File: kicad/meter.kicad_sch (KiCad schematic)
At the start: 10 parts, among them U10 MAX7219, U9 MAX7219

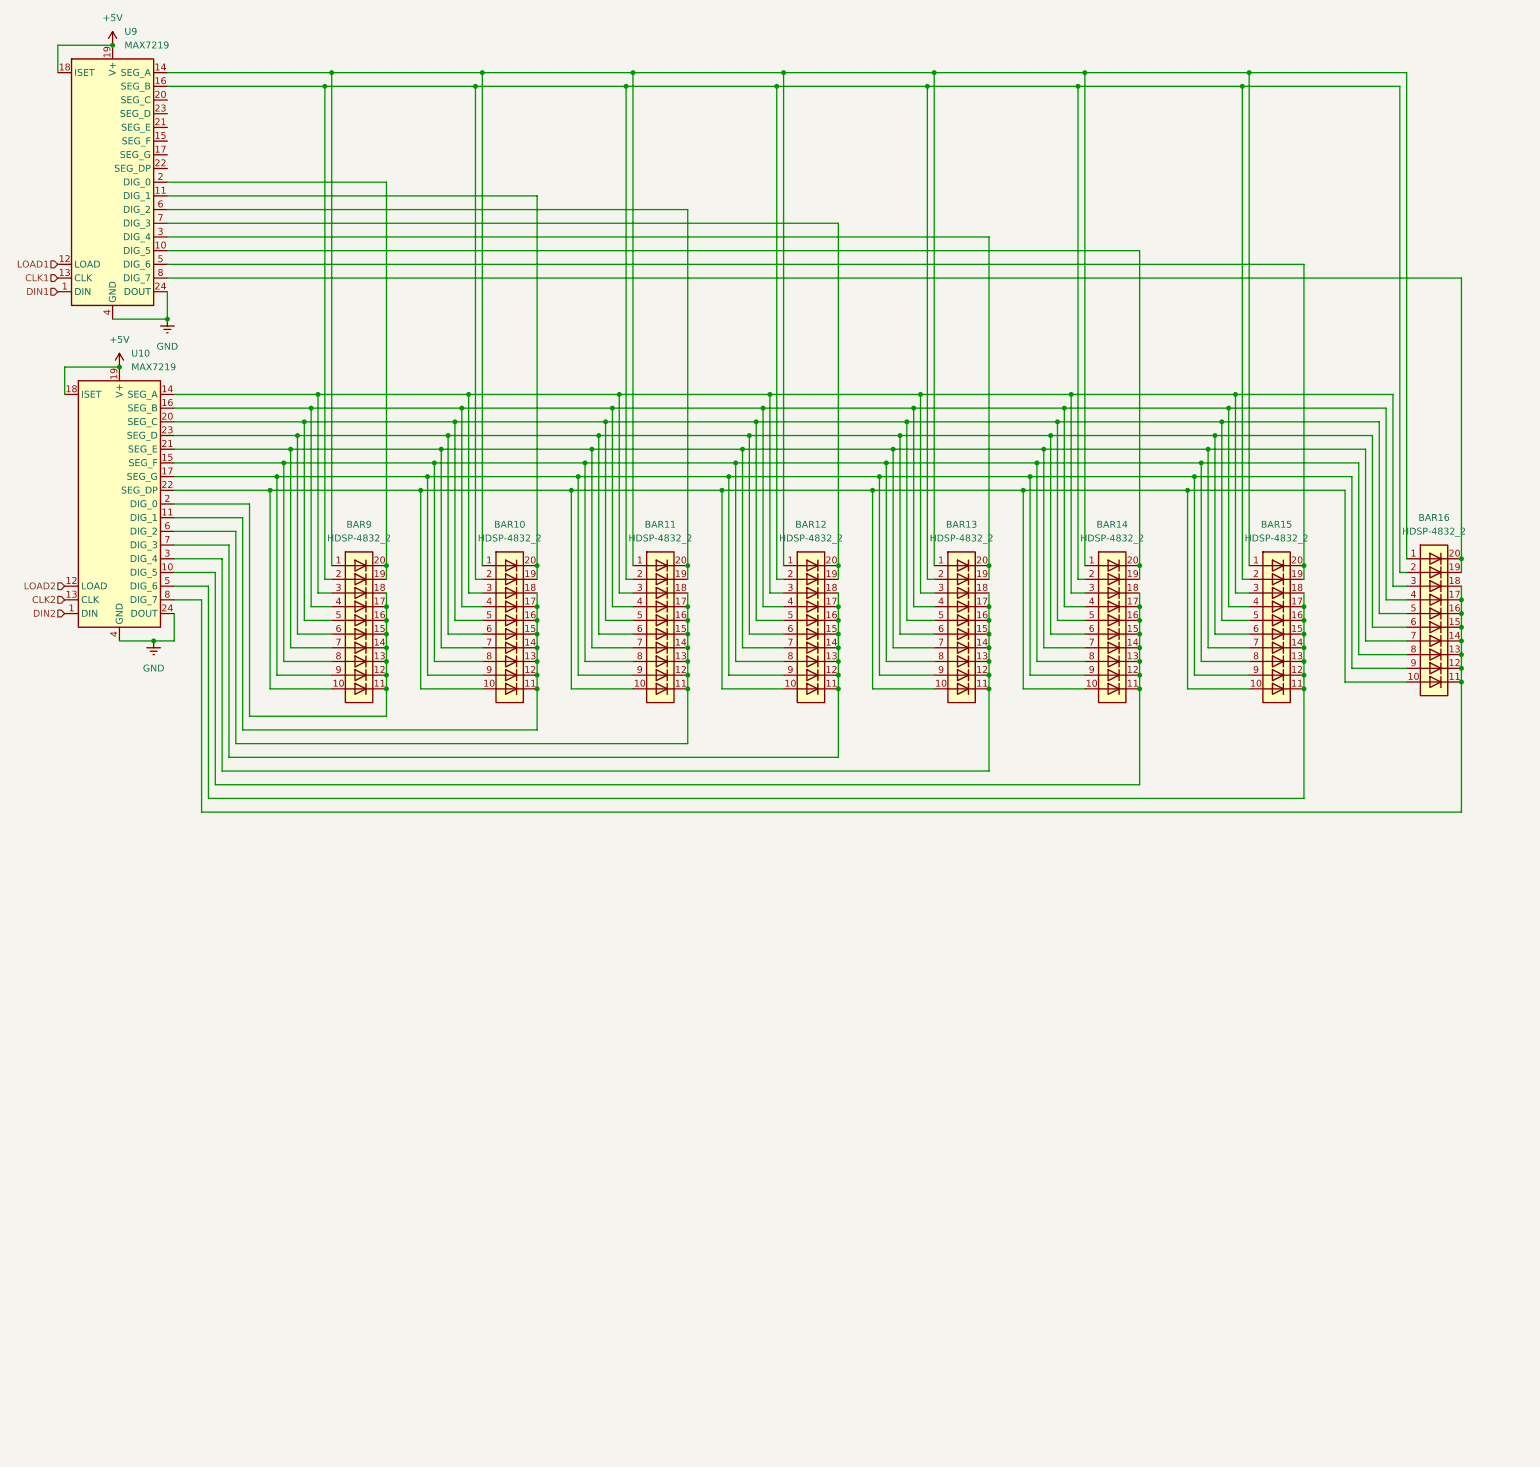
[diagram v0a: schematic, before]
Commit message: kicad updates
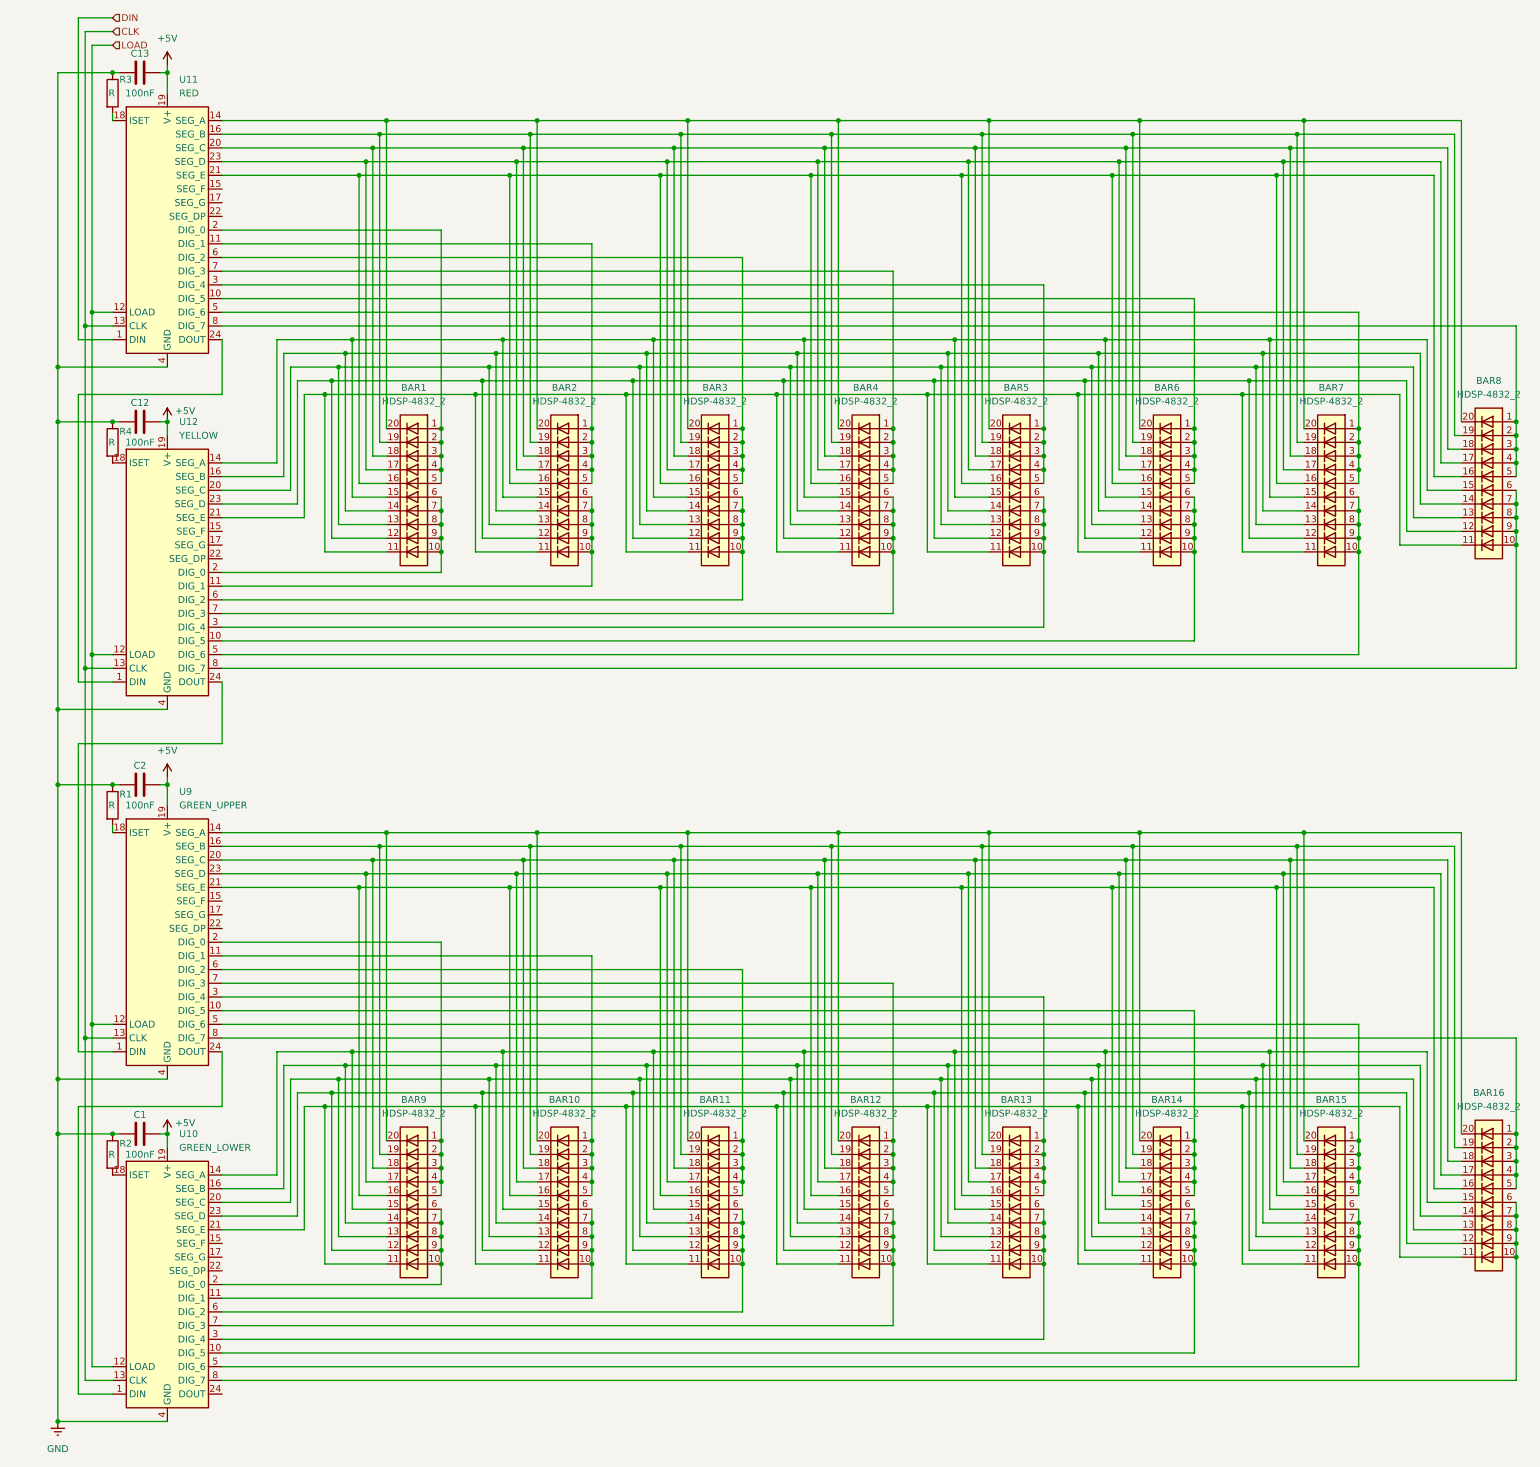
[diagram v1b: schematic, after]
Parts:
- added BAR1, BAR2, BAR3, BAR4, BAR5, BAR6, BAR7, BAR8: HDSP-4832_2, Display:HDSP-4832, symbol LED:HDSP-4832_2
- added C1, C12, C13, C2: 100nF, Capacitor_THT:C_Axial_L5.1mm_D3.1mm_P7.50mm_Horizontal, symbol Device:C
- added R1, R2, R3, R4: R, Resistor_THT:R_Axial_DIN0207_L6.3mm_D2.5mm_P10.16mm_Horizontal, symbol Device:R
- added U11: RED, Package_DIP:DIP-24_W7.62mm_Socket, symbol Driver_LED:MAX7219
- added U12: YELLOW, Package_DIP:DIP-24_W7.62mm_Socket, symbol Driver_LED:MAX7219
- U10: value MAX7219 -> GREEN_LOWER; footprint (none) -> Package_DIP:DIP-24_W7.62mm_Socket
- U9: value MAX7219 -> GREEN_UPPER; footprint (none) -> Package_DIP:DIP-24_W7.62mm_Socket
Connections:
- net CLK2 is gone; now on net CLK: U10.13 (CLK)
- net LOAD2 is gone; now on net LOAD: U10.12 (LOAD)
- net +5V: now also C1.2, C12.2, C13.2, C2.2, U11.19 (V+), U12.19 (V+); no longer U10.18 (ISET), U9.18 (ISET)
- net GND: now also C1.1, C12.1, C13.1, C2.1, R1.1, R2.1, R3.1, R4.1, U11.4 (GND), U11.9 (GND), U12.4 (GND), U12.9 (GND); no longer U10.24 (DOUT), U9.24 (DOUT)
- net at U9.20 (SEG_C): now also BAR10.18 (K), BAR11.18 (K), BAR12.18 (K), BAR13.18 (K), BAR14.18 (K), BAR15.18 (K), BAR16.18 (K), BAR9.18 (K)
- net at U9.21 (SEG_E): now also BAR10.16 (K), BAR11.16 (K), BAR12.16 (K), BAR13.16 (K), BAR14.16 (K), BAR15.16 (K), BAR16.16 (K), BAR9.16 (K)
- net at U9.23 (SEG_D): now also BAR10.17 (K), BAR11.17 (K), BAR12.17 (K), BAR13.17 (K), BAR14.17 (K), BAR15.17 (K), BAR16.17 (K), BAR9.17 (K)
- net CLK1 renamed CLK
- net CLK: now also U11.13 (CLK), U12.13 (CLK)
- net DIN1: no longer names the net of U9.1 (DIN)
- net DIN1: now also U12.24 (DOUT)
- net DIN2: no longer names the net of U10.1 (DIN)
- net DIN2: now also U9.24 (DOUT)
- net LOAD1 renamed LOAD
- net LOAD: now also U11.12 (LOAD), U12.12 (LOAD)
- new net: BAR14.10 (A), BAR14.6 (A), BAR14.7 (A), BAR14.8 (A), BAR14.9 (A), U10.10 (DIG_5)
- new net: BAR10.10 (A), BAR10.6 (A), BAR10.7 (A), BAR10.8 (A), BAR10.9 (A), U10.11 (DIG_1)
- new net: BAR10.15 (K), BAR11.15 (K), BAR12.15 (K), BAR13.15 (K), BAR14.15 (K), BAR15.15 (K), BAR16.15 (K), BAR9.15 (K), U10.14 (SEG_A)
- new net: BAR10.14 (K), BAR11.14 (K), BAR12.14 (K), BAR13.14 (K), BAR14.14 (K), BAR15.14 (K), BAR16.14 (K), BAR9.14 (K), U10.16 (SEG_B)
- new net: R2.2, U10.18 (ISET)
- new net: BAR9.10 (A), BAR9.6 (A), BAR9.7 (A), BAR9.8 (A), BAR9.9 (A), U10.2 (DIG_0)
- new net: BAR10.13 (K), BAR11.13 (K), BAR12.13 (K), BAR13.13 (K), BAR14.13 (K), BAR15.13 (K), BAR16.13 (K), BAR9.13 (K), U10.20 (SEG_C)
- new net: BAR10.11 (K), BAR11.11 (K), BAR12.11 (K), BAR13.11 (K), BAR14.11 (K), BAR15.11 (K), BAR16.11 (K), BAR9.11 (K), U10.21 (SEG_E)
- new net: BAR10.12 (K), BAR11.12 (K), BAR12.12 (K), BAR13.12 (K), BAR14.12 (K), BAR15.12 (K), BAR16.12 (K), BAR9.12 (K), U10.23 (SEG_D)
- new net: BAR13.10 (A), BAR13.6 (A), BAR13.7 (A), BAR13.8 (A), BAR13.9 (A), U10.3 (DIG_4)
- new net: BAR15.10 (A), BAR15.6 (A), BAR15.7 (A), BAR15.8 (A), BAR15.9 (A), U10.5 (DIG_6)
- new net: BAR11.10 (A), BAR11.6 (A), BAR11.7 (A), BAR11.8 (A), BAR11.9 (A), U10.6 (DIG_2)
- new net: BAR12.10 (A), BAR12.6 (A), BAR12.7 (A), BAR12.8 (A), BAR12.9 (A), U10.7 (DIG_3)
- new net: BAR16.10 (A), BAR16.6 (A), BAR16.7 (A), BAR16.8 (A), BAR16.9 (A), U10.8 (DIG_7)
- new net: BAR14.1 (A), BAR14.2 (A), BAR14.3 (A), BAR14.4 (A), BAR14.5 (A), U9.10 (DIG_5)
- new net: BAR10.1 (A), BAR10.2 (A), BAR10.3 (A), BAR10.4 (A), BAR10.5 (A), U9.11 (DIG_1)
- new net: BAR10.20 (K), BAR11.20 (K), BAR12.20 (K), BAR13.20 (K), BAR14.20 (K), BAR15.20 (K), BAR16.20 (K), BAR9.20 (K), U9.14 (SEG_A)
- new net: BAR10.19 (K), BAR11.19 (K), BAR12.19 (K), BAR13.19 (K), BAR14.19 (K), BAR15.19 (K), BAR16.19 (K), BAR9.19 (K), U9.16 (SEG_B)
- new net: R1.2, U9.18 (ISET)
- new net: BAR9.1 (A), BAR9.2 (A), BAR9.3 (A), BAR9.4 (A), BAR9.5 (A), U9.2 (DIG_0)
- new net: BAR13.1 (A), BAR13.2 (A), BAR13.3 (A), BAR13.4 (A), BAR13.5 (A), U9.3 (DIG_4)
- new net: BAR15.1 (A), BAR15.2 (A), BAR15.3 (A), BAR15.4 (A), BAR15.5 (A), U9.5 (DIG_6)
- new net: BAR11.1 (A), BAR11.2 (A), BAR11.3 (A), BAR11.4 (A), BAR11.5 (A), U9.6 (DIG_2)
- new net: BAR12.1 (A), BAR12.2 (A), BAR12.3 (A), BAR12.4 (A), BAR12.5 (A), U9.7 (DIG_3)
- new net: BAR16.1 (A), BAR16.2 (A), BAR16.3 (A), BAR16.4 (A), BAR16.5 (A), U9.8 (DIG_7)
- new net: BAR3.1 (A), BAR3.2 (A), BAR3.3 (A), BAR3.4 (A), BAR3.5 (A), U11.6 (DIG_2)
- new net: BAR3.10 (A), BAR3.6 (A), BAR3.7 (A), BAR3.8 (A), BAR3.9 (A), U12.6 (DIG_2)
- new net: BAR1.11 (K), BAR2.11 (K), BAR3.11 (K), BAR4.11 (K), BAR5.11 (K), BAR6.11 (K), BAR7.11 (K), BAR8.11 (K), U12.21 (SEG_E)
- new net: BAR1.12 (K), BAR2.12 (K), BAR3.12 (K), BAR4.12 (K), BAR5.12 (K), BAR6.12 (K), BAR7.12 (K), BAR8.12 (K), U12.23 (SEG_D)
- new net: BAR1.13 (K), BAR2.13 (K), BAR3.13 (K), BAR4.13 (K), BAR5.13 (K), BAR6.13 (K), BAR7.13 (K), BAR8.13 (K), U12.20 (SEG_C)
- new net: BAR1.14 (K), BAR2.14 (K), BAR3.14 (K), BAR4.14 (K), BAR5.14 (K), BAR6.14 (K), BAR7.14 (K), BAR8.14 (K), U12.16 (SEG_B)
- new net: BAR1.15 (K), BAR2.15 (K), BAR3.15 (K), BAR4.15 (K), BAR5.15 (K), BAR6.15 (K), BAR7.15 (K), BAR8.15 (K), U12.14 (SEG_A)
- new net: BAR1.16 (K), BAR2.16 (K), BAR3.16 (K), BAR4.16 (K), BAR5.16 (K), BAR6.16 (K), BAR7.16 (K), BAR8.16 (K), U11.21 (SEG_E)
- new net: BAR1.17 (K), BAR2.17 (K), BAR3.17 (K), BAR4.17 (K), BAR5.17 (K), BAR6.17 (K), BAR7.17 (K), BAR8.17 (K), U11.23 (SEG_D)
- new net: BAR1.18 (K), BAR2.18 (K), BAR3.18 (K), BAR4.18 (K), BAR5.18 (K), BAR6.18 (K), BAR7.18 (K), BAR8.18 (K), U11.20 (SEG_C)
- new net: BAR1.19 (K), BAR2.19 (K), BAR3.19 (K), BAR4.19 (K), BAR5.19 (K), BAR6.19 (K), BAR7.19 (K), BAR8.19 (K), U11.16 (SEG_B)
- new net: BAR1.20 (K), BAR2.20 (K), BAR3.20 (K), BAR4.20 (K), BAR5.20 (K), BAR6.20 (K), BAR7.20 (K), BAR8.20 (K), U11.14 (SEG_A)
- new net: R4.2, U12.18 (ISET)
- new net: BAR4.1 (A), BAR4.2 (A), BAR4.3 (A), BAR4.4 (A), BAR4.5 (A), U11.7 (DIG_3)
- new net: BAR4.10 (A), BAR4.6 (A), BAR4.7 (A), BAR4.8 (A), BAR4.9 (A), U12.7 (DIG_3)
- new net: BAR6.1 (A), BAR6.2 (A), BAR6.3 (A), BAR6.4 (A), BAR6.5 (A), U11.10 (DIG_5)
- new net: BAR6.10 (A), BAR6.6 (A), BAR6.7 (A), BAR6.8 (A), BAR6.9 (A), U12.10 (DIG_5)
- new net: BAR2.1 (A), BAR2.2 (A), BAR2.3 (A), BAR2.4 (A), BAR2.5 (A), U11.11 (DIG_1)
- new net: R3.2, U11.18 (ISET)
- new net: BAR1.1 (A), BAR1.2 (A), BAR1.3 (A), BAR1.4 (A), BAR1.5 (A), U11.2 (DIG_0)
- new net: U11.24 (DOUT), U12.1 (DIN)
- new net: BAR5.1 (A), BAR5.2 (A), BAR5.3 (A), BAR5.4 (A), BAR5.5 (A), U11.3 (DIG_4)
- new net: BAR7.1 (A), BAR7.2 (A), BAR7.3 (A), BAR7.4 (A), BAR7.5 (A), U11.5 (DIG_6)
- new net: BAR8.1 (A), BAR8.2 (A), BAR8.3 (A), BAR8.4 (A), BAR8.5 (A), U11.8 (DIG_7)
- new net: BAR2.10 (A), BAR2.6 (A), BAR2.7 (A), BAR2.8 (A), BAR2.9 (A), U12.11 (DIG_1)
- new net: BAR1.10 (A), BAR1.6 (A), BAR1.7 (A), BAR1.8 (A), BAR1.9 (A), U12.2 (DIG_0)
- new net: BAR5.10 (A), BAR5.6 (A), BAR5.7 (A), BAR5.8 (A), BAR5.9 (A), U12.3 (DIG_4)
- new net: BAR7.10 (A), BAR7.6 (A), BAR7.7 (A), BAR7.8 (A), BAR7.9 (A), U12.5 (DIG_6)
- new net: BAR8.10 (A), BAR8.6 (A), BAR8.7 (A), BAR8.8 (A), BAR8.9 (A), U12.8 (DIG_7)
- new net DIN: U11.1 (DIN)
- now unconnected: U10.15 (SEG_F), U10.17 (SEG_G), U10.22 (SEG_DP)
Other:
- moved on the sheet: BAR10, BAR11, BAR12, BAR13, BAR14, BAR15, BAR16, BAR9, U10, U9
